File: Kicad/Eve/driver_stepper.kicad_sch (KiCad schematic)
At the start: 19 parts, among them J201 Conn_01x04, Q201 SQJ504EP-T1_GE3, Q202 SQJ504EP-T1_GE3, Q203 SQJ504EP-T1_GE3, Q204 SQJ504EP-T1_GE3, U201 TMC2590-TA

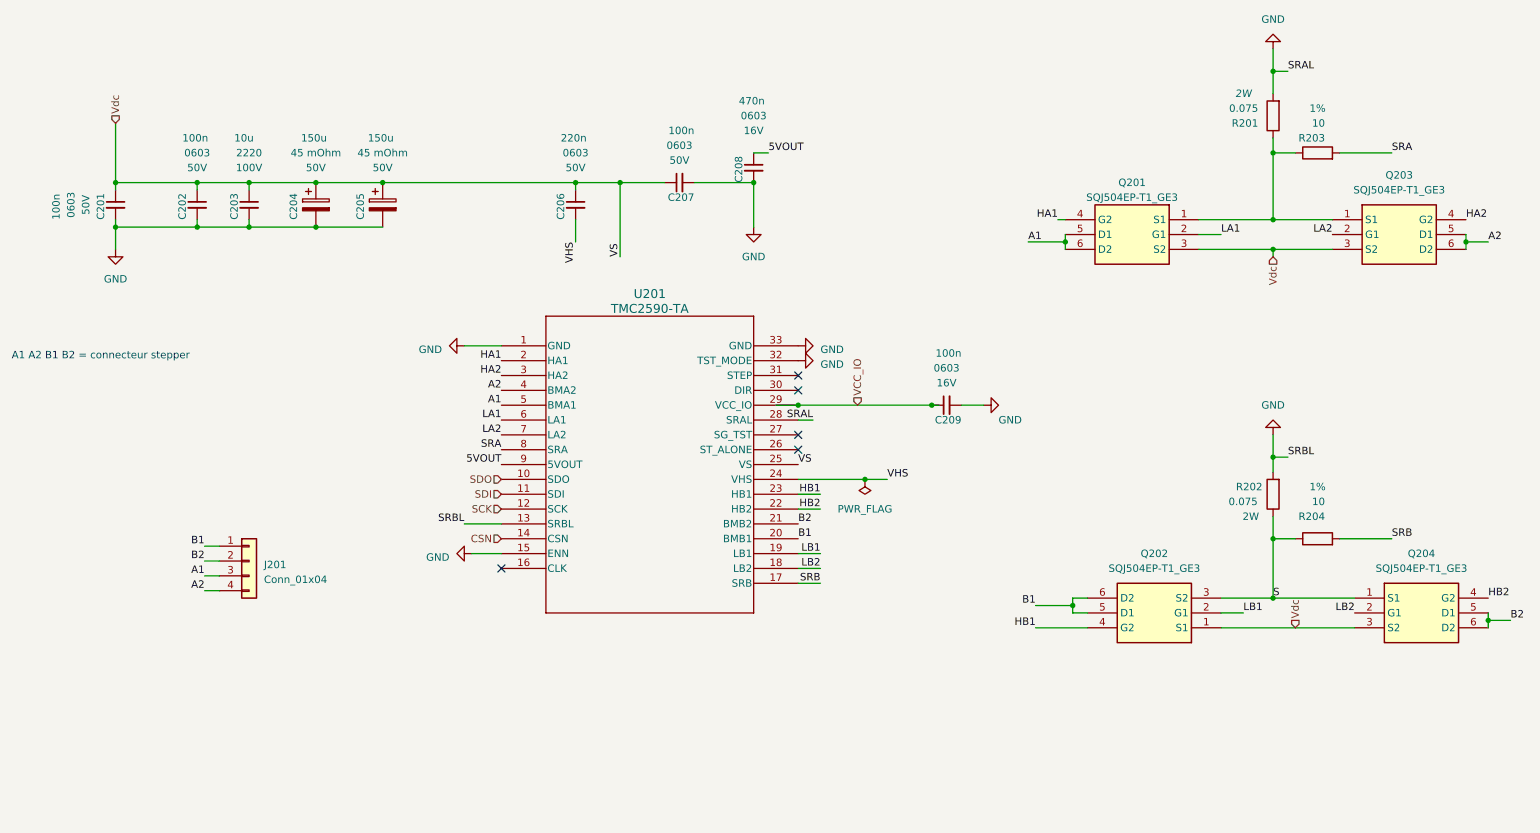
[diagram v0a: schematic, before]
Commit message: update pcb
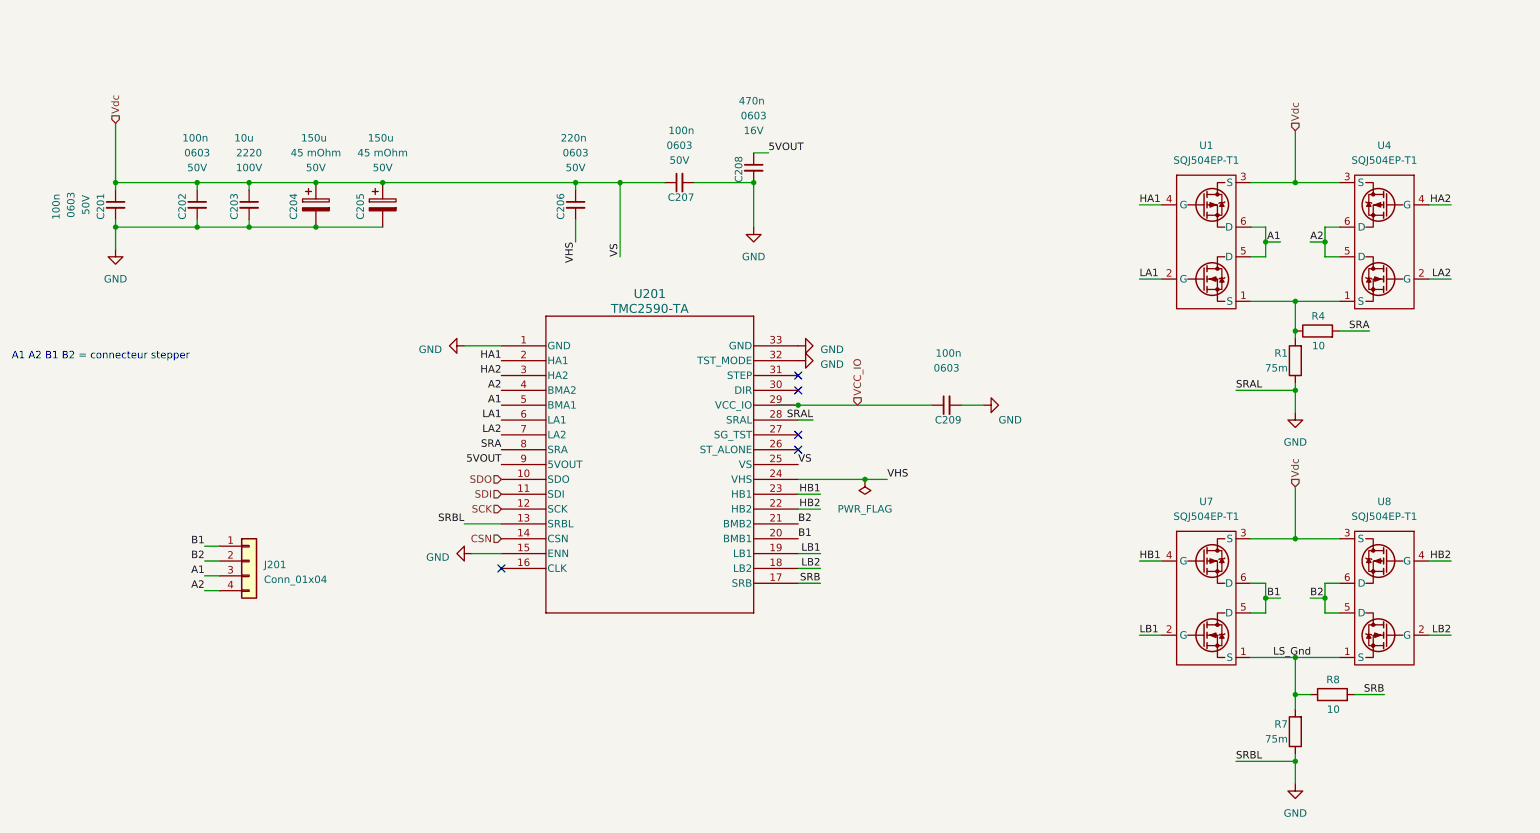
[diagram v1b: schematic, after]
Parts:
- removed Q201, Q202, Q203, Q204: SQJ504EP-T1_GE3, Mosfet:SQJ968EPT1GE3, symbol SQJ504EP-T1_GE3:SQJ504EP-T1_GE3
- removed R201, R202: 0.075, Resistor_SMD:R_2512_6332Metric, symbol Device:R
- removed R203, R204: 10, Resistor_SMD:R_0402_1005Metric, symbol Device:R
- added R1, R7: 75m, Resistor_SMD:R_2512_6332Metric, symbol Device:R
- added R4, R8: 10, Resistor_SMD:R_0402_1005Metric, symbol Device:R
- added U1, U4, U7, U8: SQJ504EP-T1, Mosfet:SQJ968EPT1GE3, symbol SQJ504EP-T1:SQJ504EP-T1_GE3
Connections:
- net A1: now also U1.5 (D), U1.6 (D)
- net A2: now also U4.5 (D), U4.6 (D)
- net B1: now also U7.5 (D), U7.6 (D)
- net B2: now also U8.5 (D), U8.6 (D)
- net GND: now also R1.1, R7.1
- net HA1: now also U1.4 (G)
- net HA2: now also U4.4 (G)
- net HB1: now also U7.4 (G)
- net HB2: now also U8.4 (G)
- net LA1: now also U1.2 (G)
- net LA2: now also U4.2 (G)
- net LB1: now also U7.2 (G)
- net LB2: now also U8.2 (G)
- net SRA: now also R4.2
- net SRB: now also R8.2
- net Vdc: now also U1.3 (S), U4.3 (S), U7.3 (S), U8.3 (S)
- new net: R1.2, R4.1, U1.1 (S), U4.1 (S)
- new net LS_Gnd: R7.2, R8.1, U7.1 (S), U8.1 (S)
